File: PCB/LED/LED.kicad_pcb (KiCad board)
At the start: 2 copper layers, 11.5 x 28.7 mm, 22 parts, among them J1 Conn_01x03, J2 USB-C, J3 Shelly, Q1 PMF170XP,115, Q2 PMF250XNEX, U1 ESP32-PICO-MINI-02, U2 QR, U3 LMR16006XDDCR

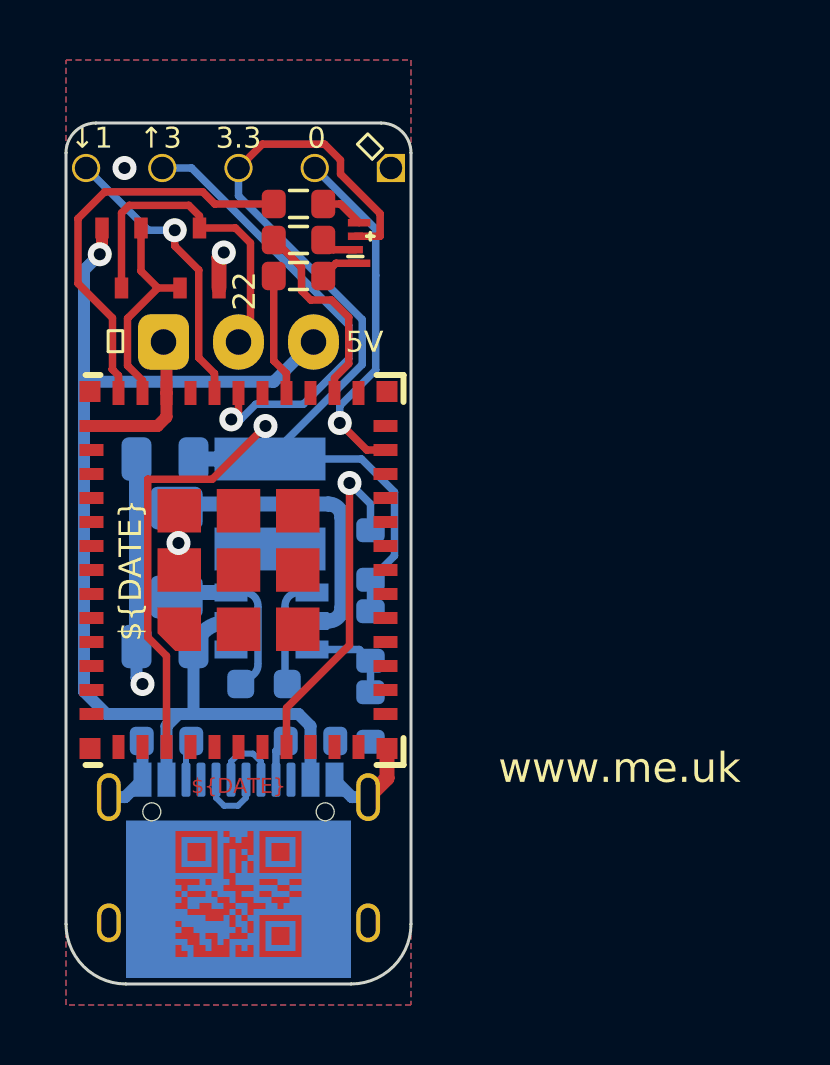
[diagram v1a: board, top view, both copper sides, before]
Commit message: New PCB
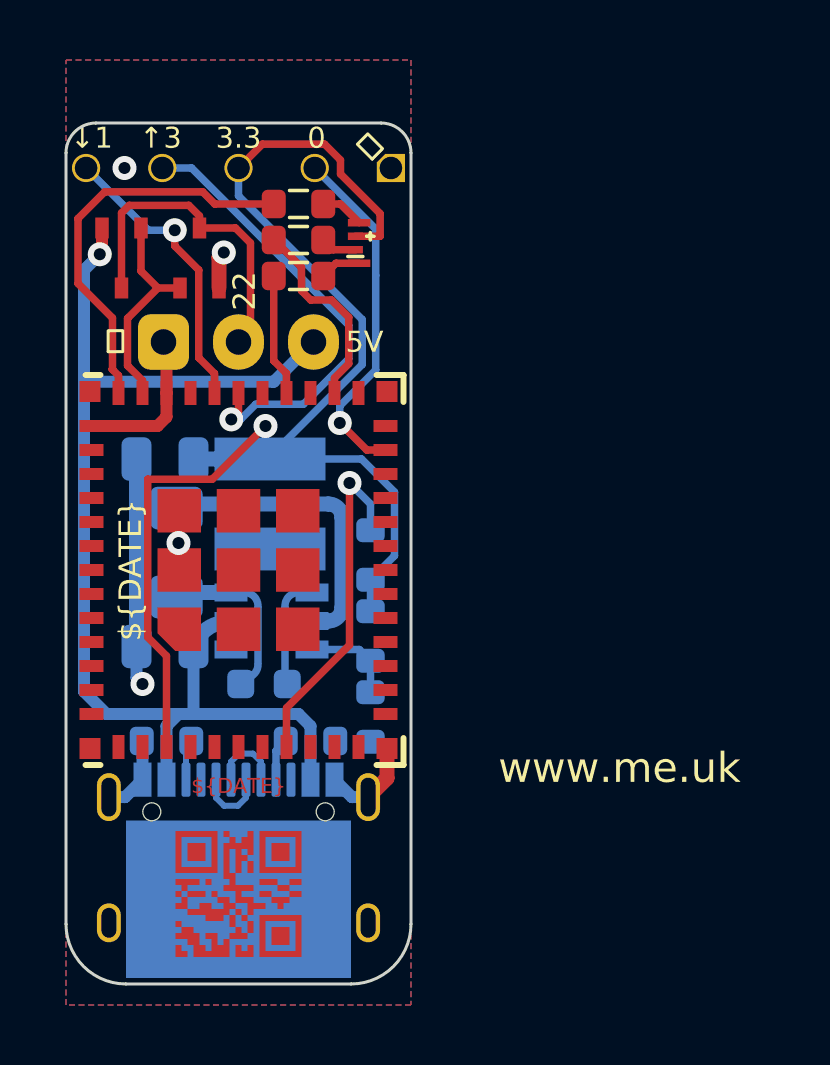
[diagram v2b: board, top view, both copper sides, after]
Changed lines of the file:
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@@
     (at 101.1 99.2 90)
     (descr "LMR16006 based fixed regulator")
-    (property "JLCPCB Rotation Offset" "90")
-    (property "LCSC Part #" "C87080")
+    (property "JLCPCB Rotation Offset" "180")
+    (property "LCSC Part #" "C290195")
     (property "Manufacturer" "TI")
     (property "Part No" "LMR16006XDDCR")
@@
       (options (clearance outline) (anchor rect))
       (primitives
-    (gr_arc (start 0.001745 0.000002) (mid 0.707106 0.292893) (end 0.999998 0.998254) (width 0.5))
+    (gr_arc (start 0.001745 0.000002) (mid 0.705871 0.29166) (end 0.999986 0.994764) (width 0.5))
       ))
     (pad "5" smd roundrect (at -0.85 -2.6 180) (size 1 1.45) (layers "B.Cu" "B.Paste" "B.Mask") (roundrect_rratio 0.25)
@@
     (descr "USB Type C CMT R/A PCB  Mount Socket 16pin Power+Data")
     (tags "USB-C")
+    (property "JLCPCB Rotation Offset" "180")
     (property "LCSC Part #" "C709357")
     (property "Sheetfile" "LED.kicad_sch")
